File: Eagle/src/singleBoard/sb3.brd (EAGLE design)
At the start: 82.5 x 97.3 mm, 39 parts, among them J1 UJ2-BH-1-TH, Q2 IRFD9120, U1 GY-521MPU6050

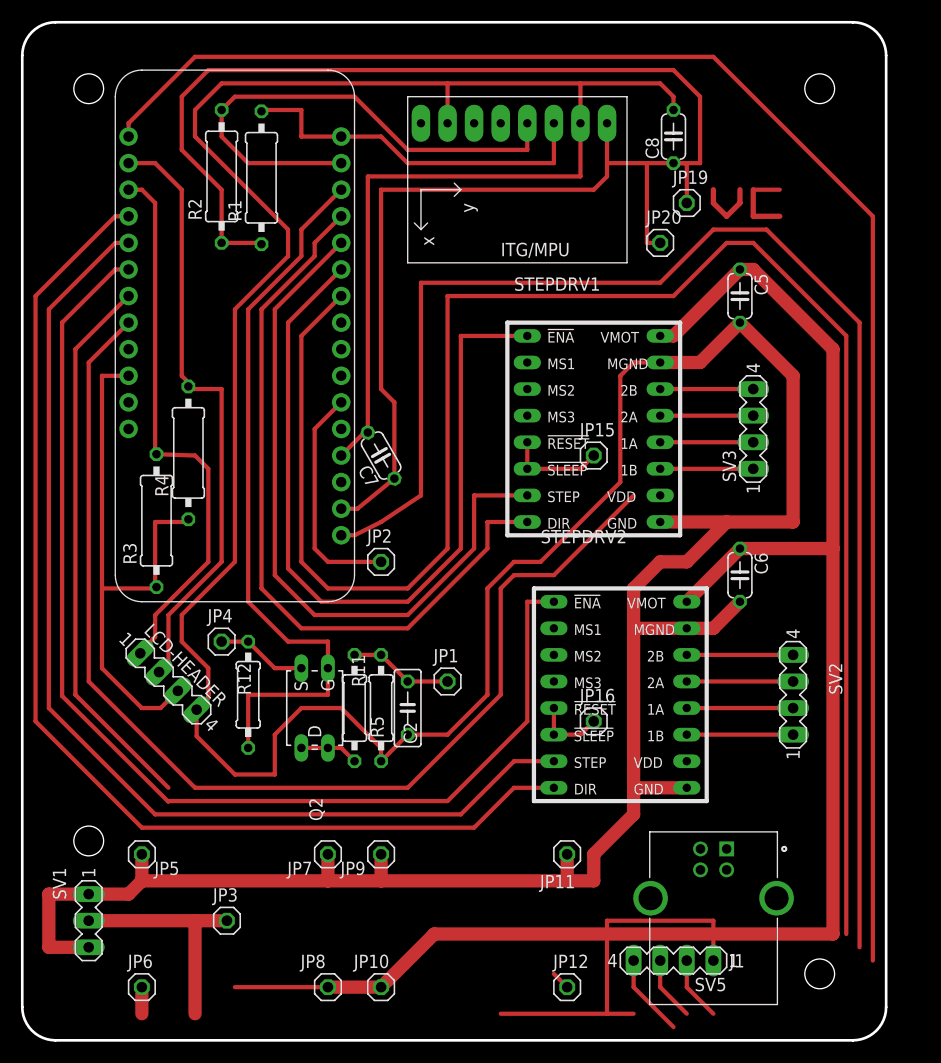
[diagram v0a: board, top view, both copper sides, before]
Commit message: finalization of single board design, plus remoted switches and usb jack
finalization of single board design, plus remoted switches and usb jack
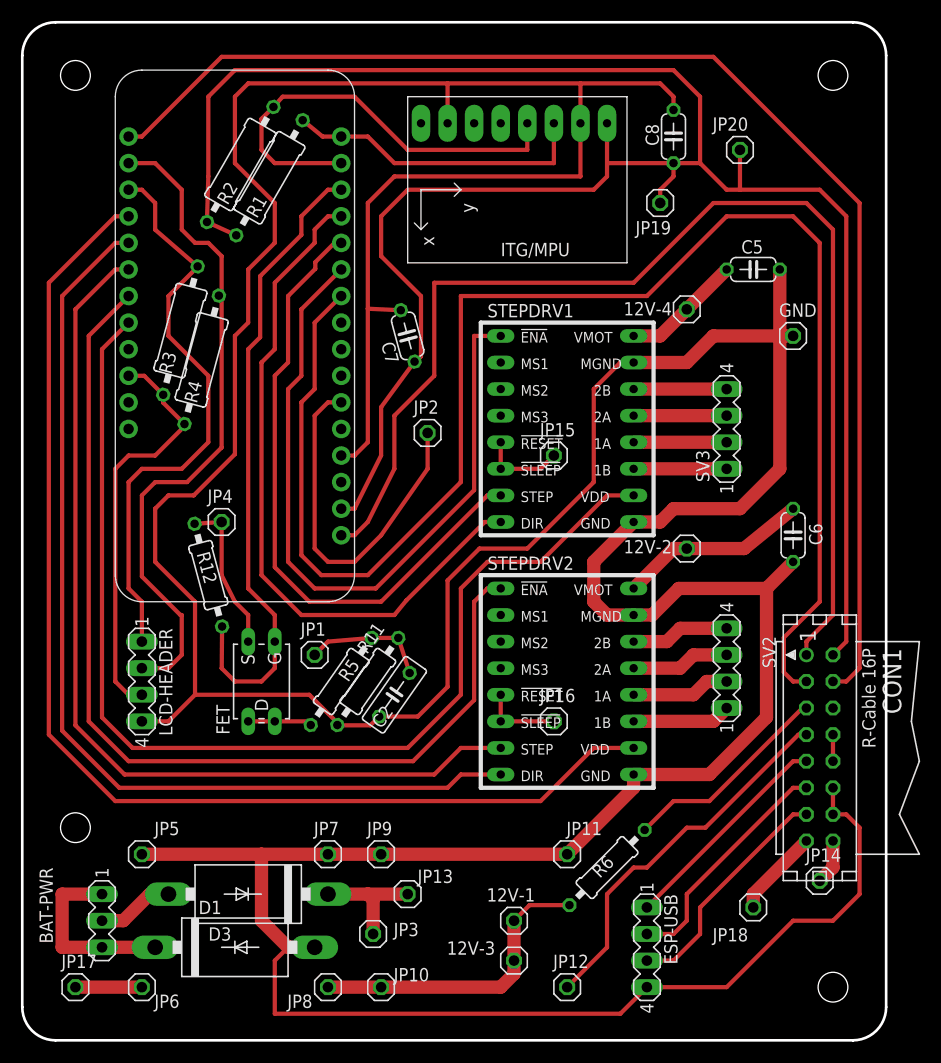
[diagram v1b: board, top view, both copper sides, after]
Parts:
- removed J1: UJ2-BH-1-TH, UJ2-BH-1-TH:CUI_UJ2-BH-1-TH
- removed Q2: IRFD9120, transistor-small-signal:C370-01
- removed SV1: (no value), con-lstb:MA03-1
- removed SV5: (no value), con-lstb:MA04-1
- added 12V-1, 12V-2, 12V-3, 12V-4, GND, JP13, JP14, JP17, JP18: (no value), pinhead:1X01
- added BAT-PWR: (no value), con-lstb:MA03-1
- added CON1: (no value), con-harting:CON16
- added D1, D3: 1N5400, diode:DO201-15
- added ESP-USB: (no value), con-lstb:MA04-1
- added FET: IRFD9120, transistor-small-signal:C370-01
- added R6: (no value), rcl:0207/10
- moved R3 18.3 mm to (15.1, 67.8), turned to 75 degrees
- moved JP3 14.0 mm to (33.5, 10.2)
- moved JP2 13.1 mm to (38.7, 58.0)
- moved JP1 13.0 mm to (27.9, 36.8)
- moved R12 12.0 mm to (17.8, 44.5), turned to 285 degrees
- moved C7 11.7 mm to (36.8, 67.3), turned to 105 degrees
- moved JP20 11.7 mm to (68.6, 85.1)
- moved JP4 11.4 mm to (19.1, 49.5)
- moved R4 8.98 mm to (17.1, 65.0), turned to 75 degrees
- moved SV2 6.84 mm to (67.3, 35.6)
- moved C6 6.35 mm to (73.7, 48.3)
- moved STEPDRV2 5.24 mm to (53.3, 35.6)
- moved JP15 3.81 mm to (50.8, 55.9)
- moved JP16 3.81 mm to (50.8, 30.5)
- moved R5 2.84 mm to (30.5, 34.3), turned to 235 degrees
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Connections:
- removed net N$39: SV5.4
- removed net N$48: SV5.1
- removed net N$56: J1.1
- removed net VDD: STEPDRV1.10, STEPDRV2.10
- new net N$1: MS2.24, STEPDRV1.10
- new net N$2: CON1.5, R6.2
- new net N$26: BAT-PWR.2, D1.A
- new net N$42: 12V-1.1, 12V-3.1, JP10.1, JP8.1, R6.1
- new net N$43: CON1.7, JP12.1
- new net N$44: 12V-2.1, C6.1, STEPDRV2.16
- new net N$46: BAT-PWR.1, BAT-PWR.3, D3.C
- new net N$55: CON1.9, ESP-USB.1
- net 3V: now also CON1.2
- net N$22: now also CON1.11, ESP-USB.2; no longer J1.2, SV5.2
- net N$23: now also CON1.13, ESP-USB.3; no longer J1.3, SV5.3
- net N$24: now also FET.S; no longer Q2.S
- net N$27: now also JP17.1, JP6.1; no longer MS2.20, STEPDRV2.8
- net N$28: now also CON1.4
- net N$29: now also STEPDRV2.8; no longer STEPDRV2.7
- net N$31: now also CON1.3
- net N$32: now also D1.C, JP13.1; no longer SV1.2
- net N$34: now also STEPDRV2.7; no longer STEPDRV2.1
- net N$36: now also MS2.20, STEPDRV2.10; no longer MS2.23
- net N$37: now also MS2.23, STEPDRV2.1; no longer MS2.24
- net N$38: now also CON1.15, JP18.1; no longer JP6.1
- net N$4: now also CON1.1
- net N$40: now also CON1.10, CON1.8; no longer J1.4, J1.SH1, J1.SH2
- net N$41: now also C2.1, C5.2, C6.2, C7.2, C8.2, CON1.12, CON1.14, D3.A, ESP-USB.4, GND.1, JP11.1, JP5.1, JP7.1, JP9.1, LCD-HEADER.4, MS2.4, R11.1, STEPDRV1.15, STEPDRV1.9, STEPDRV2.15, STEPDRV2.9, U1.ADO, U1.GND; no longer C5.1, C6.1, JP10.1, JP8.1, STEPDRV1.16, STEPDRV2.16
- net N$45: now also 12V-4.1, C5.1, STEPDRV1.16; no longer JP12.1
- net N$51: now also FET.D, FET.D1; no longer Q2.D, Q2.D1
- net N$6: now also FET.G; no longer Q2.G
- net N$9: now also CON1.16, JP14.1; no longer C2.1, C5.2, C6.2, C7.2, C8.2, JP11.1, JP5.1, JP7.1, JP9.1, LCD-HEADER.4, MS2.4, R11.1, STEPDRV1.15, STEPDRV1.9, STEPDRV2.15, STEPDRV2.9, SV1.1, SV1.3, U1.ADO, U1.GND
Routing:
- net N$9: track 432.2 -> 4.34 mm
- net N$41: track 153.5 -> 501.1 mm
- net N$27: track 108.0 -> 6.35 mm
- net N$1: track 6.13 -> 106.7 mm
- net N$36: track 52.8 -> 114.0 mm
- net 3V: track 161.8 -> 207.2 mm
- net N$43: track 0.00 -> 35.8 mm
- net N$48: track 35.6 -> 0.00 mm
- net N$42: track 0.00 -> 29.3 mm
- net N$28: track 152.5 -> 126.3 mm
- net N$4: track 136.4 -> 112.1 mm
- net N$31: track 168.7 -> 147.3 mm
- net N$55: track 0.00 -> 21.0 mm
- net N$2: track 0.00 -> 20.3 mm
- net N$34: track 109.9 -> 90.0 mm
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
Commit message: upload from Doug's PC
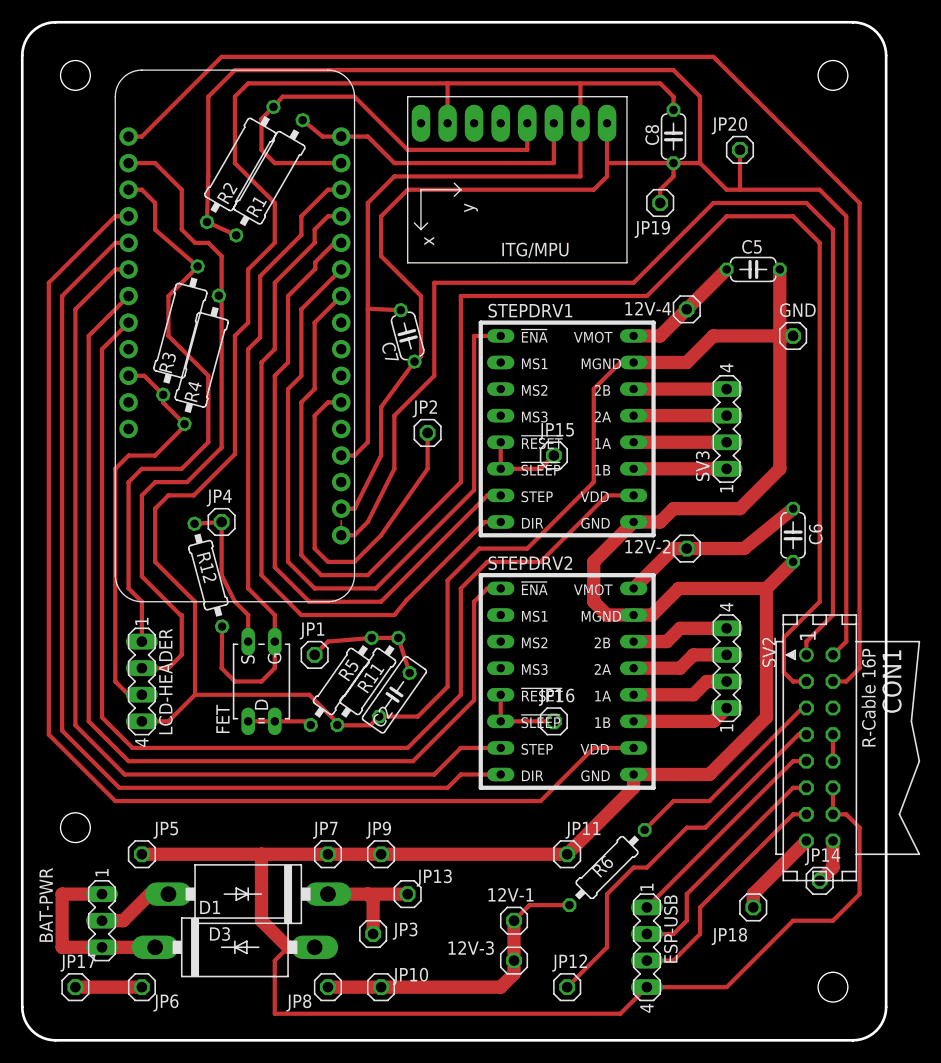
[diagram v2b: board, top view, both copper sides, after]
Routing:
- net N$4: track 112.1 -> 113.5 mm
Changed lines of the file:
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@@
 </layers>
 <board>
-<fusionsync huburn="a.cGVyc29uYWw6dWUyZDlmNmRl" projecturn="a.cGVyc29uYWw6dWUyZDlkNTAxIzIwMTgxMDI0MTU2NDI4OTAx" f3durn="urn:adsk.wipprod:dm.lineage:RVMtdEYxSvOPFW49h7ULsg" pcbguid="49d98df1-49b2-45fb-9c3f-6a5aa2b8ca4d" lastpulledtime="2019-02-27T19:32:19Z" lastsyncedchangeguid="2b95e2a0-3dcb-4e46-8abe-5d507ab46a9a"/>
+<fusionsync huburn="a.cGVyc29uYWw6dWUyZDlmNmRl" projecturn="a.cGVyc29uYWw6dWUyZDlkNTAxIzIwMTgxMDI0MTU2NDI4OTAx" f3durn="urn:adsk.wipprod:dm.lineage:RVMtdEYxSvOPFW49h7ULsg" pcbguid="49d98df1-49b2-45fb-9c3f-6a5aa2b8ca4d" lastpulledtime="2019-03-17T19:19:13Z" lastsyncedchangeguid="24049744-be62-3583-beae-4fb7246fa9cf"/>
 <plain>
 <dimension x1="0" y1="118.11" x2="82.55" y2="118.11" x3="41.275" y3="120.65" textsize="1.778" layer="1" unit="inch"/>
 <dimension x1="-7.62" y1="0" x2="-7.62" y2="96.52" x3="-8.89" y3="48.26" textsize="1.778" layer="1" unit="inch"/>
-<hole x="77.47" y="92.202" drill="2.8448"/>
-<hole x="5.08" y="20.32" drill="2.8448"/>
-<hole x="5.08" y="92.202" drill="2.8448"/>
-<hole x="77.47" y="5.08" drill="2.8448"/>
+<hole x="77.47" y="92.202" drill="2.845"/>
+<hole x="5.08" y="20.32" drill="2.845"/>
+<hole x="5.08" y="92.202" drill="2.845"/>
+<hole x="77.47" y="5.08" drill="2.845"/>
 <wire x1="82.55" y1="94.107" x2="79.375" y2="97.282" width="0.254" layer="20" curve="90"/>
 <wire x1="79.375" y1="97.282" x2="3.175" y2="97.282" width="0.254" layer="20"/>
@@
 </element>
 <element name="R11" library="rcl" library_urn="urn:adsk.eagle:library:334" package="0207/10" package3d_urn="urn:adsk.eagle:package:23491/1" value="" x="33.02" y="34.29" smashed="yes" rot="R55">
-<attribute name="NAME" x="32.93711875" y="36.828646875" size="1.27" layer="25" ratio="10" rot="R55"/>
+<attribute name="NAME" x="32.93711875" y="33.018646875" size="1.27" layer="25" ratio="10" rot="R55"/>
 <attribute name="SPICEPREFIX" value="R" x="106.876459375" y="-63.9363625" size="1.778" layer="27" rot="R55" display="off"/>
 <attribute name="VALUE" x="106.09999375" y="-66.15235625" size="1.27" layer="27" ratio="10" rot="R55"/>
@@
 <wire x1="30.48" y1="50.8" x2="31.75" y2="50.8" width="0.4064" layer="1"/>
 <wire x1="31.75" y1="50.8" x2="34.29" y2="55.88" width="0.4064" layer="1"/>
-<wire x1="34.29" y1="60.49931875" x2="34.29" y2="55.88" width="0.4064" layer="1"/>
+<wire x1="34.29" y1="55.88" x2="34.29" y2="60.49931875" width="0.4064" layer="1"/>
 <wire x1="37.4874" y1="64.856546875" x2="34.29" y2="60.49931875" width="0.4064" layer="1"/>
 <wire x1="17.78" y1="82.55" x2="17.643903125" y2="78.11904375" width="0.4064" layer="1"/>
@@
 <contactref element="CON1" pad="1"/>
 <wire x1="74.93" y1="38.1" x2="74.93" y2="36.83" width="0.4064" layer="1"/>
+<wire x1="30.48" y1="48.26" x2="30.48" y2="49.6824" width="0.1524" layer="1"/>
 </signal>
 <signal name="N$3">

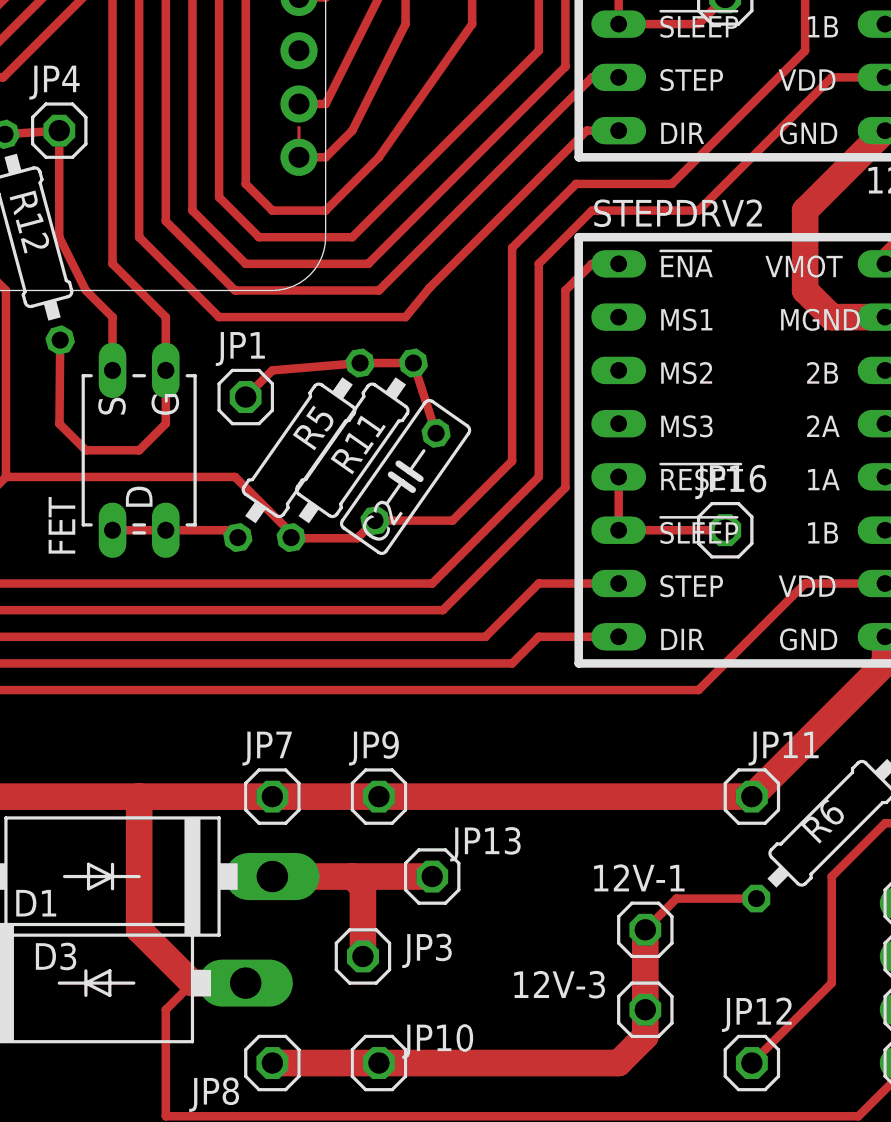
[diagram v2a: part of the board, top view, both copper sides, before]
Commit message: final fixesbefore release to manufacturing
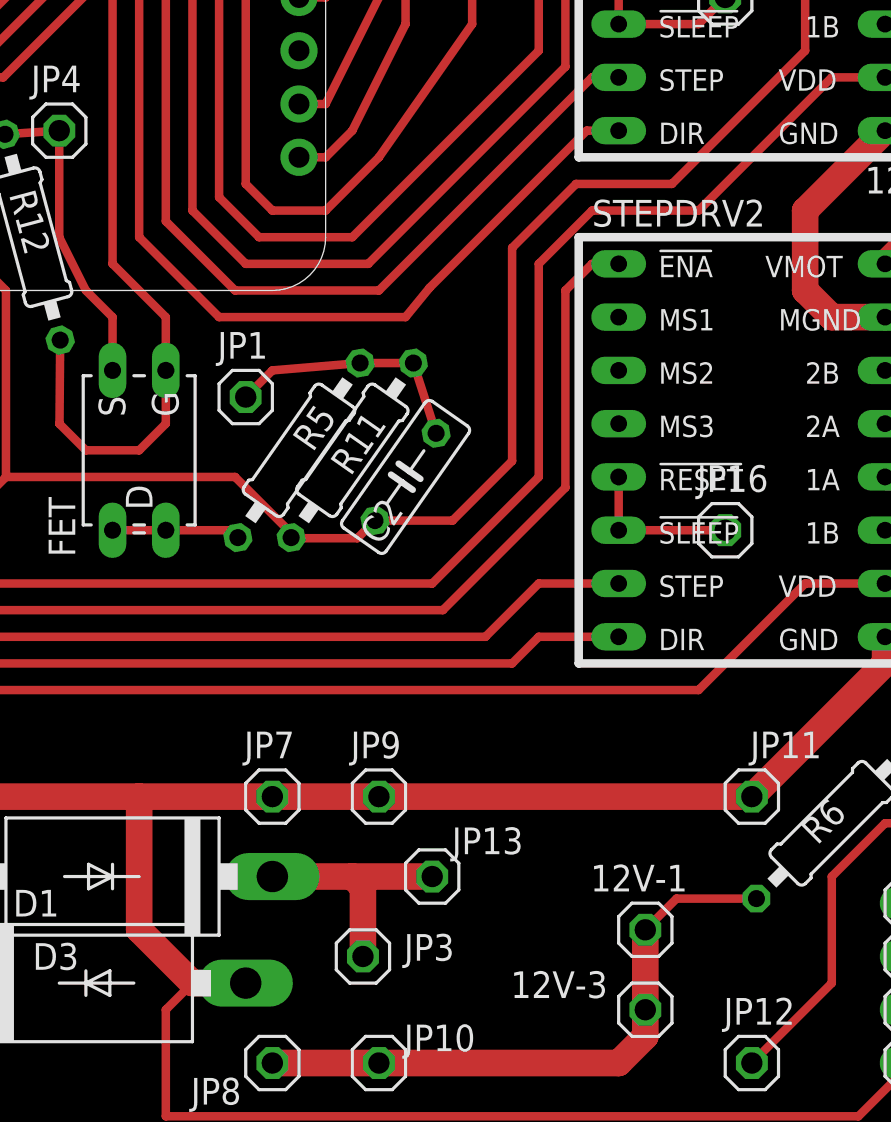
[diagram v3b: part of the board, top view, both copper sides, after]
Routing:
- net N$4: track 113.5 -> 112.1 mm

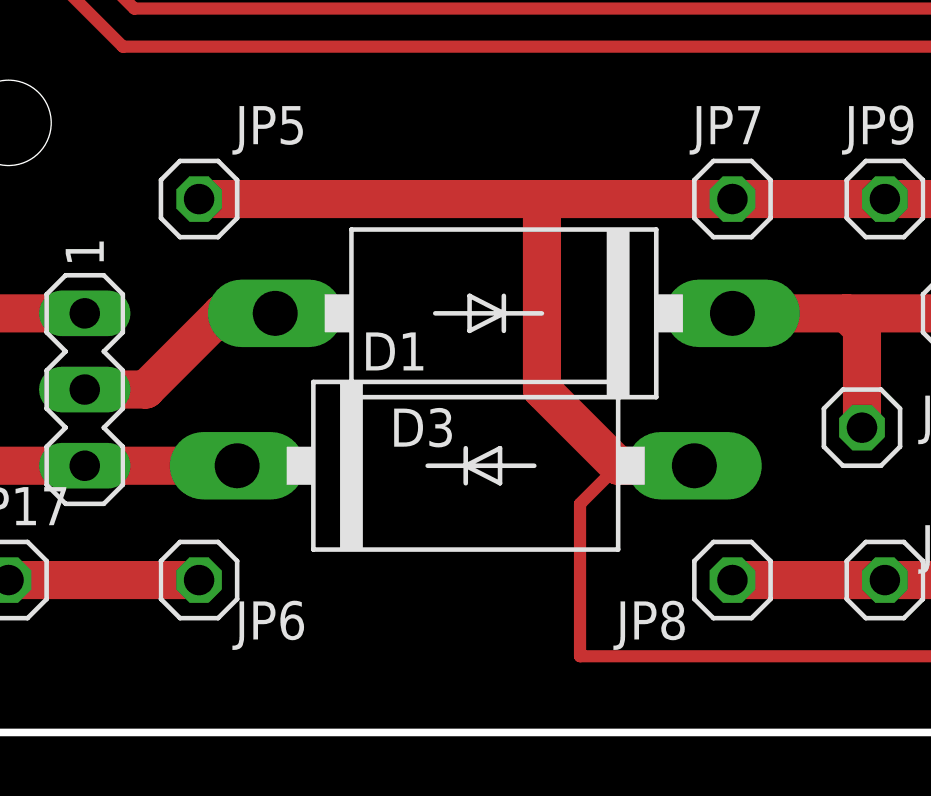
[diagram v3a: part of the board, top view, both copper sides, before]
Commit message: trivial change to force update
this file has length 171,438
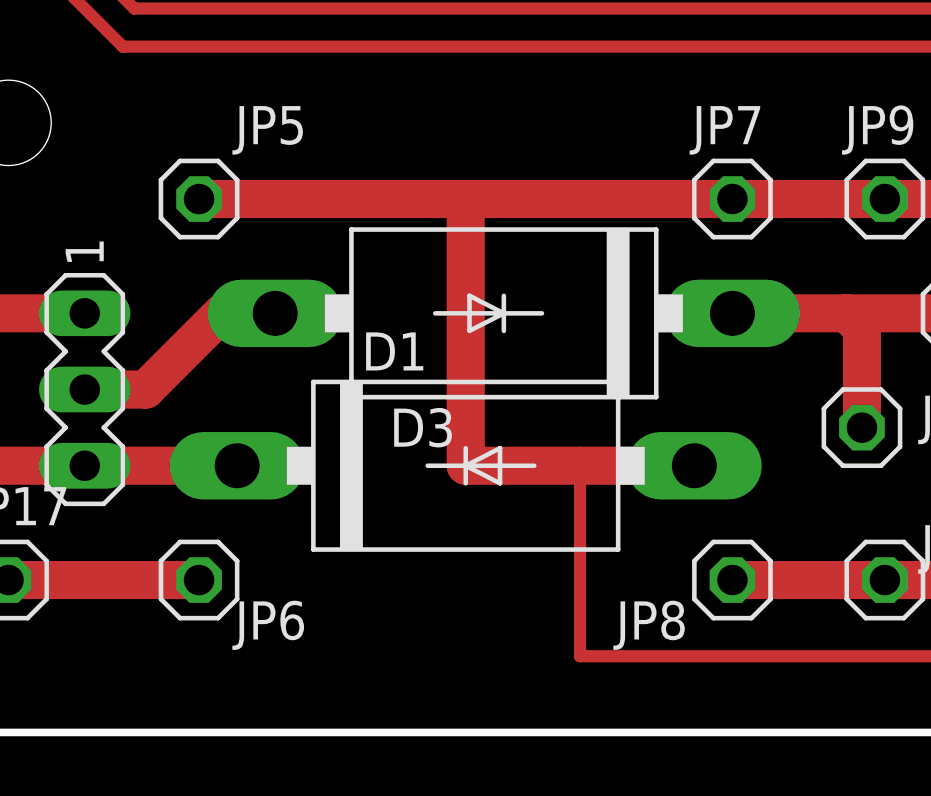
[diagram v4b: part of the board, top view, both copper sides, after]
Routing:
- net N$39: track 501.1 -> 504.6 mm
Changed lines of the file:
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@@
 <?xml version="1.0" encoding="utf-8"?>
 <!DOCTYPE eagle SYSTEM "eagle.dtd">
-<eagle version="9.3.0">
+<eagle version="9.4.0">
 <drawing>
 <settings>
@@
 <wire x1="60.96" y1="49.53" x2="62.23" y2="50.8" width="1.27" layer="1"/>
 <wire x1="54.61" y1="45.72" x2="58.42" y2="49.53" width="1.27" layer="1"/>
-<wire x1="25.4" y1="8.89" x2="24.13" y2="7.62" width="0.4064" layer="1"/>
-<wire x1="24.13" y1="7.62" x2="24.13" y2="2.54" width="0.4064" layer="1"/>
+<wire x1="24.13" y1="8.89" x2="24.13" y2="2.54" width="0.4064" layer="1"/>
 <wire x1="57.15" y1="2.54" x2="24.13" y2="2.54" width="0.4064" layer="1"/>
 <wire x1="59.69" y1="5.08" x2="57.15" y2="2.54" width="0.4064" layer="1"/>
@@
 <wire x1="80.01" y1="13.97" x2="80.01" y2="20.32" width="0.4064" layer="1"/>
 <wire x1="67.31" y1="5.08" x2="73.66" y2="11.43" width="0.4064" layer="1"/>
-<wire x1="25.4" y1="8.89" x2="22.86" y2="11.43" width="1.27" layer="1"/>
-<wire x1="22.86" y1="17.78" x2="22.86" y2="11.43" width="1.27" layer="1"/>
+<wire x1="20.32" y1="17.78" x2="20.32" y2="8.89" width="1.27" layer="1"/>
 <wire x1="16.51" y1="33.02" x2="27.432" y2="33.02" width="0.4064" layer="1"/>
 <wire x1="16.51" y1="33.02" x2="13.97" y2="30.48" width="0.4064" layer="1"/>
@@
 <wire x1="57.15" y1="64.77" x2="54.61" y2="62.23" width="0.4064" layer="1"/>
 <wire x1="55.88" y1="40.64" x2="54.61" y2="41.91" width="1.27" layer="1"/>
-<wire x1="11.43" y1="17.78" x2="22.86" y2="17.78" width="1.27" layer="1"/>
-<wire x1="22.86" y1="17.78" x2="29.21" y2="17.78" width="1.27" layer="1"/>
+<wire x1="11.43" y1="17.78" x2="20.32" y2="17.78" width="1.27" layer="1"/>
+<wire x1="20.32" y1="17.78" x2="29.21" y2="17.78" width="1.27" layer="1"/>
 <wire x1="29.21" y1="17.78" x2="34.29" y2="17.78" width="1.27" layer="1"/>
 <wire x1="34.29" y1="17.78" x2="52.07" y2="17.78" width="1.27" layer="1"/>
-<wire x1="25.4" y1="8.89" x2="27.94" y2="8.89" width="1.27" layer="1"/>
+<wire x1="20.32" y1="8.89" x2="24.13" y2="8.89" width="1.27" layer="1"/>
+<wire x1="24.13" y1="8.89" x2="27.94" y2="8.89" width="1.27" layer="1"/>
 </signal>
 </signals>
